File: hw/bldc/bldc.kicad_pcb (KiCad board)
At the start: 2 copper layers, 54 x 29 mm, 71 parts, among them IC1 MP2315SGJ-P, J1 Conn_01x05, J3 Conn_01x06, Q1 BSC13DN30NSFD, Q10 BSC13DN30NSFD, Q2 BSC13DN30NSFD, Q7 BSC13DN30NSFD, Q8 BSC13DN30NSFD, Q9 BSC13DN30NSFD, U1 LD1117S33TR_SOT223, U2 IR2101, U3 IR2101, U4 IR2101, U5 STM32L431CCTx

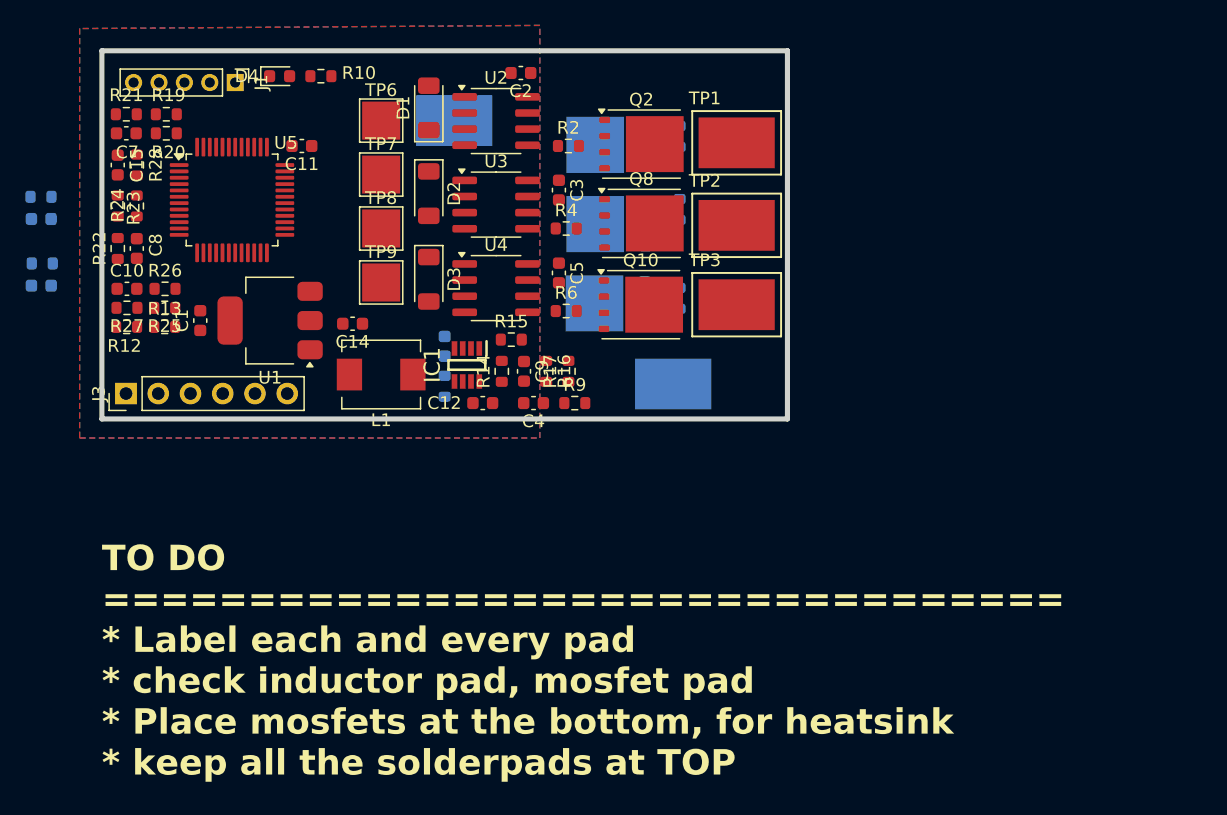
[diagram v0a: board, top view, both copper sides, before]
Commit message: pcb routing update
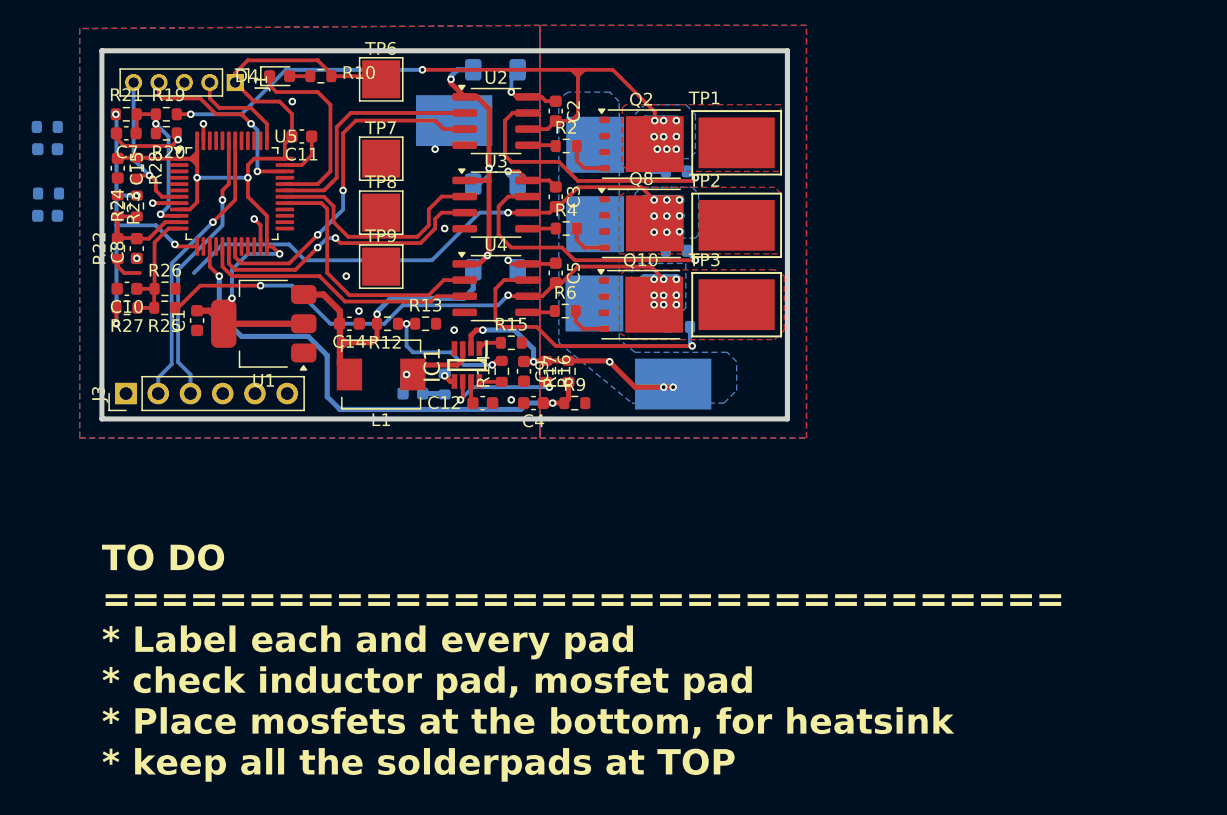
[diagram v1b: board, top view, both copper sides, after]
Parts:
- D1, D2, D3: moved to B.Cu
- moved R12 20.6 mm to (72.5, 117.5)
- moved R13 20.6 mm to (75.5, 117.5)
- moved D1 6.05 mm to (81.0, 97.5), turned to 180 degrees
- moved C16 5.52 mm to (45.7, 103.8)
- moved C17 5.52 mm to (45.7, 109.0)
- moved R18 5.52 mm to (45.8, 107.2)
- moved R7 5.52 mm to (45.7, 102.0)
- moved D2 5.30 mm to (81.0, 106.5), turned to 180 degrees
- moved D3 5.30 mm to (81.0, 113.2), turned to 180 degrees
- moved C13 4.49 mm to (74.5, 123.0), turned to 180 degrees
- moved C2 4.07 mm to (85.8, 100.8), turned to -90 degrees
- moved R3 3.26 mm to (95.2, 111.8), turned to 180 degrees
- moved TP6 3.25 mm to (72.0, 98.2)
- moved R1 2.76 mm to (95.2, 105.5), turned to 180 degrees
- moved R5 2.25 mm to (95.5, 117.8), turned to 180 degrees
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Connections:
- U2 pad 2: /TIM1_CH1 -> /TIM1_CH3
- U2 pad 3: /TIM1_CH1N -> /TIM1_CH3N
- U4 pad 2: /TIM1_CH3 -> /TIM1_CH1
- U4 pad 3: /TIM1_CH3N -> /TIM1_CH1N
- U5 pad 28: /LED -> unconnected-(U5-PB15-Pad28)
- U5 pad 32: unconnected-(U5-PA11-Pad32) -> /LED
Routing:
- net +3V3: track 0.00 -> 69.6 mm, vias 0 -> 4
- net /PHASE_A: track 0.00 -> 62.6 mm, vias 0 -> 11
- net /PHASE_B: track 0.00 -> 53.7 mm, vias 0 -> 10
- net /PHASE_C: track 0.00 -> 52.8 mm, vias 0 -> 11
- net VDD: track 0.00 -> 51.7 mm, vias 0 -> 4
- net /ADC_VDC: track 0.00 -> 40.6 mm, vias 0 -> 2
- net /TIM1_CH3N: track 0.00 -> 27.6 mm, vias 0 -> 2
- net /ADC_CENTER: track 0.00 -> 26.5 mm, vias 0 -> 4
- net Net-(U4-HO): track 0.00 -> 23.2 mm, vias 0 -> 1
- net /TIM1_CH2N: track 0.00 -> 22.8 mm, vias 0 -> 2
- net /MCU_TX: track 0.00 -> 22.4 mm, vias 0 -> 1
- net Net-(U3-HO): track 0.00 -> 22.2 mm, vias 0 -> 1
- net /TIM1_CH1N: track 0.00 -> 22.0 mm
- net /MCU_RX: track 0.00 -> 22.0 mm, vias 0 -> 1
- net Net-(U2-HO): track 0.00 -> 21.6 mm, vias 0 -> 1
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- added copper zone on B.Cu, net /PHASE_A
- added copper zone on F.Cu, net /PHASE_A
- added copper zone on B.Cu, net /PHASE_B
- added copper zone on F.Cu, net /PHASE_B
- added copper zone on B.Cu, net /PHASE_C
- added copper zone on F.Cu, net /PHASE_C
- added copper zone on B.Cu, net VDC
